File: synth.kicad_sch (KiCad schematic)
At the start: 4 parts, among them U1 ${SIM.PARAMS}

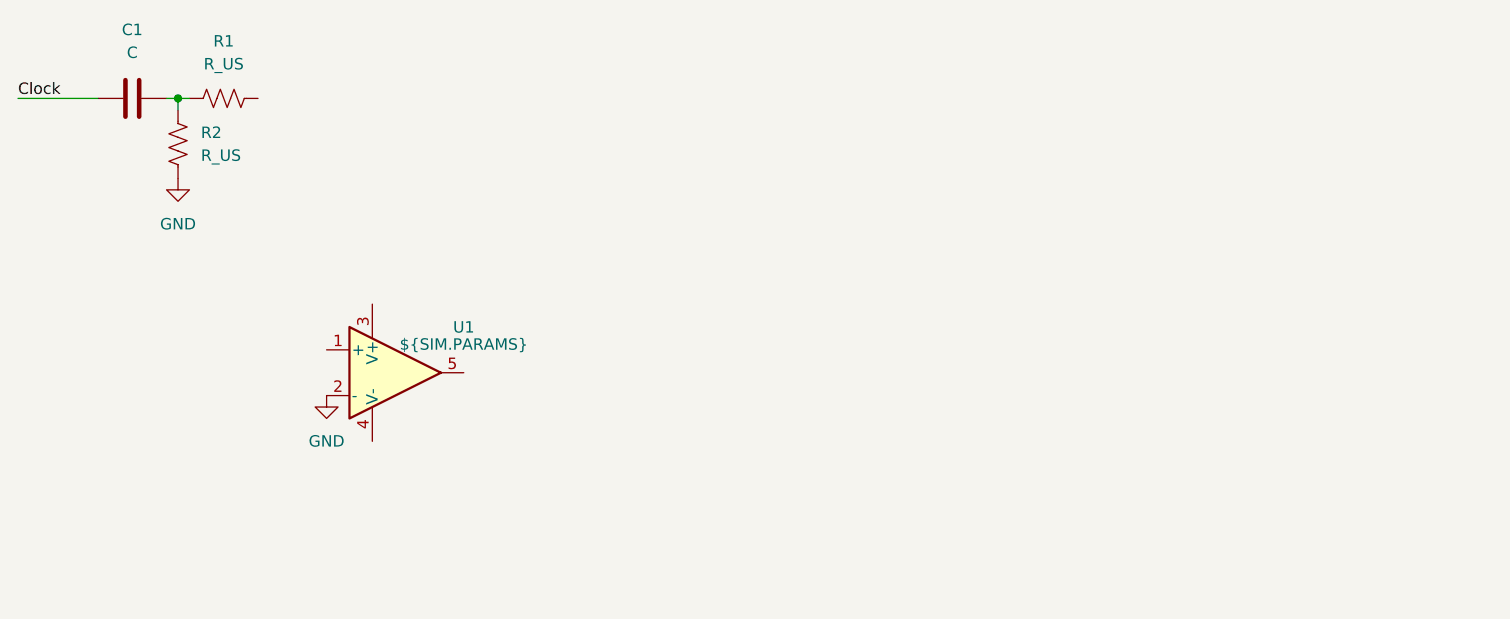
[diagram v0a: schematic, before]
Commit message: Oscilator
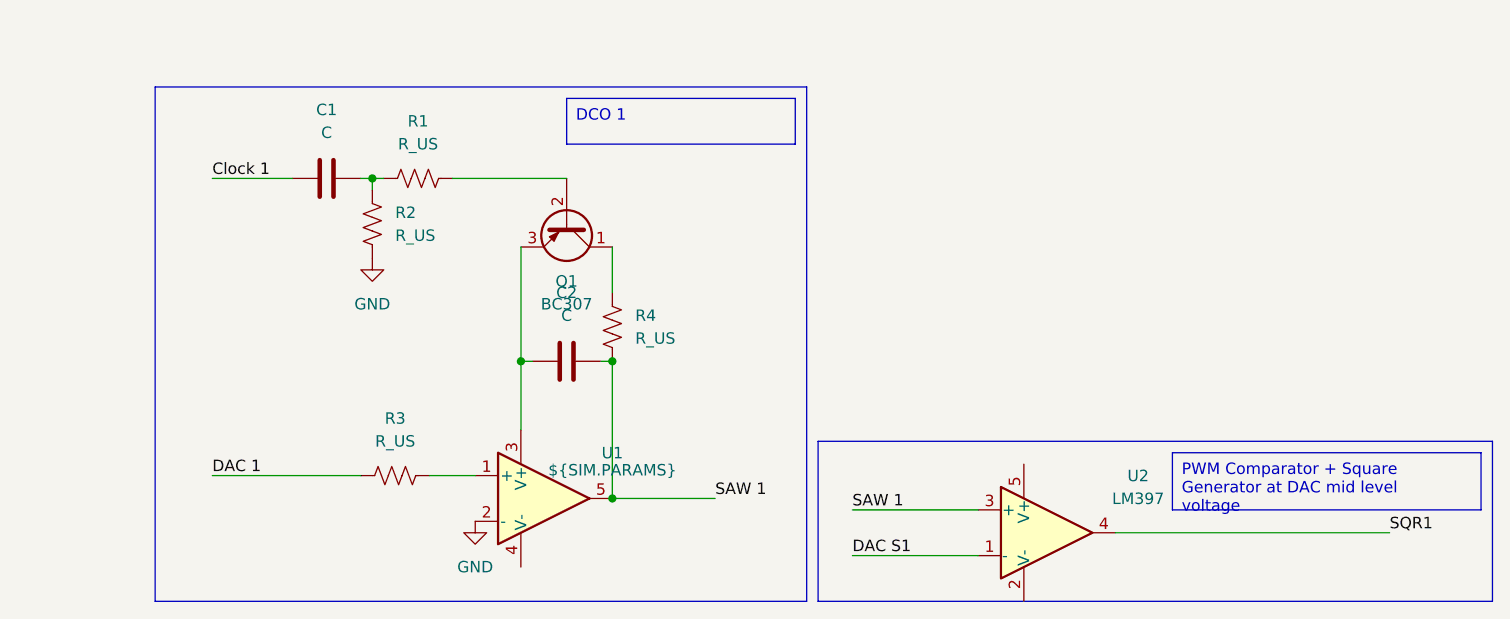
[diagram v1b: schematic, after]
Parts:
- added C2: C, symbol Device:C
- added Q1: BC307, Package_TO_SOT_THT:TO-92_Inline, symbol Transistor_BJT:BC307
- added R3, R4: R_US, symbol Device:R_US
- added U2: LM397, Package_TO_SOT_SMD:SOT-23-5, symbol Comparator:LM397
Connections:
- net at U1.1 (+): now also R3.2
- net at U1.3 (V+): now also C2.1, Q1.3 (E)
- net SAW 1: now reaches U1.5
- net SAW 1: now also C2.2, R4.1, U2.3 (+)
- net at R1.2: now also Q1.2 (B)
- net Clock renamed Clock 1
- new net: Q1.1 (C), R4.2
- new net DAC 1: R3.1
- new net DAC S1: U2.1 (-)
- new net SQR1: U2.4
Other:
- moved on the sheet: C1, R1, R2, U1
